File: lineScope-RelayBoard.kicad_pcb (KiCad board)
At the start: 2 copper layers, 99.5 x 38 mm, 18 parts, among them J10 Conn_01x03, J2 Conn_01x02, K1 RM85-1011-35-1012, K2 RM85-1011-35-1012, K3 RM85-1011-35-1012

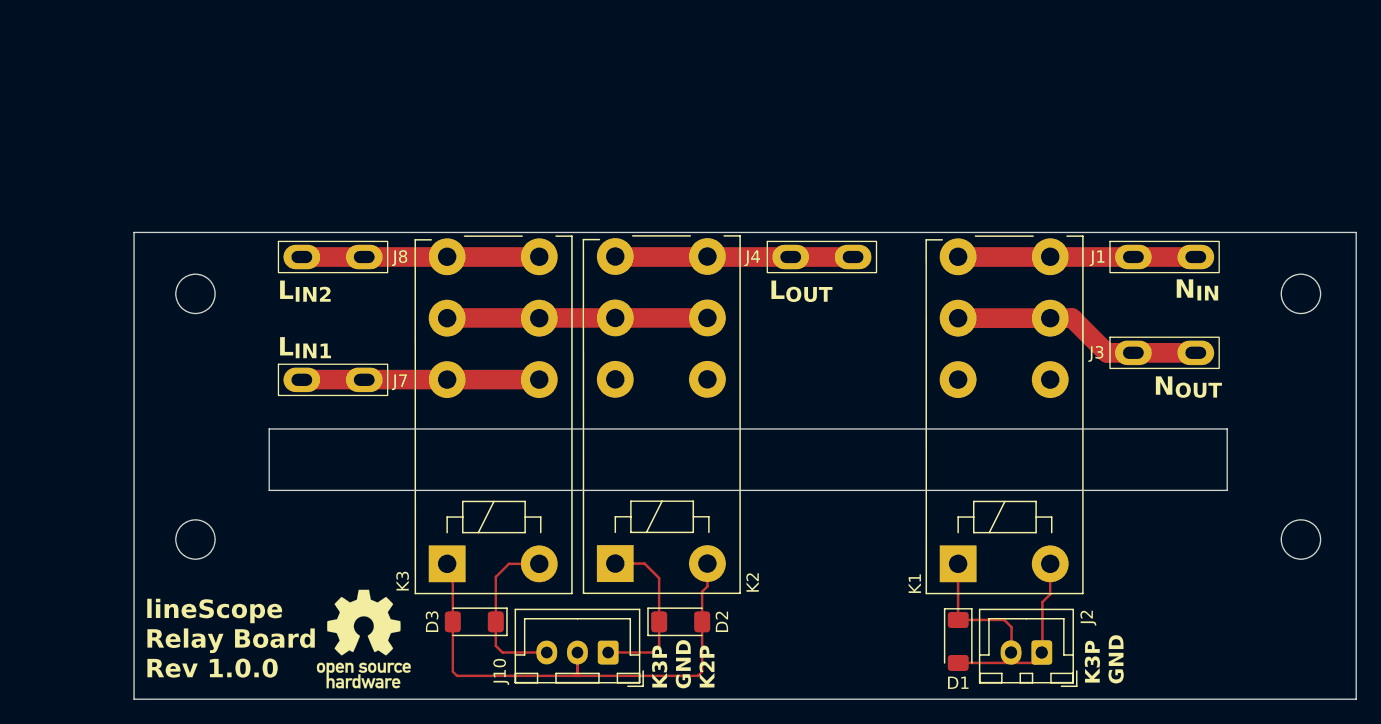
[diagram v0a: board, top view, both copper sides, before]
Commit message: Minor fixes
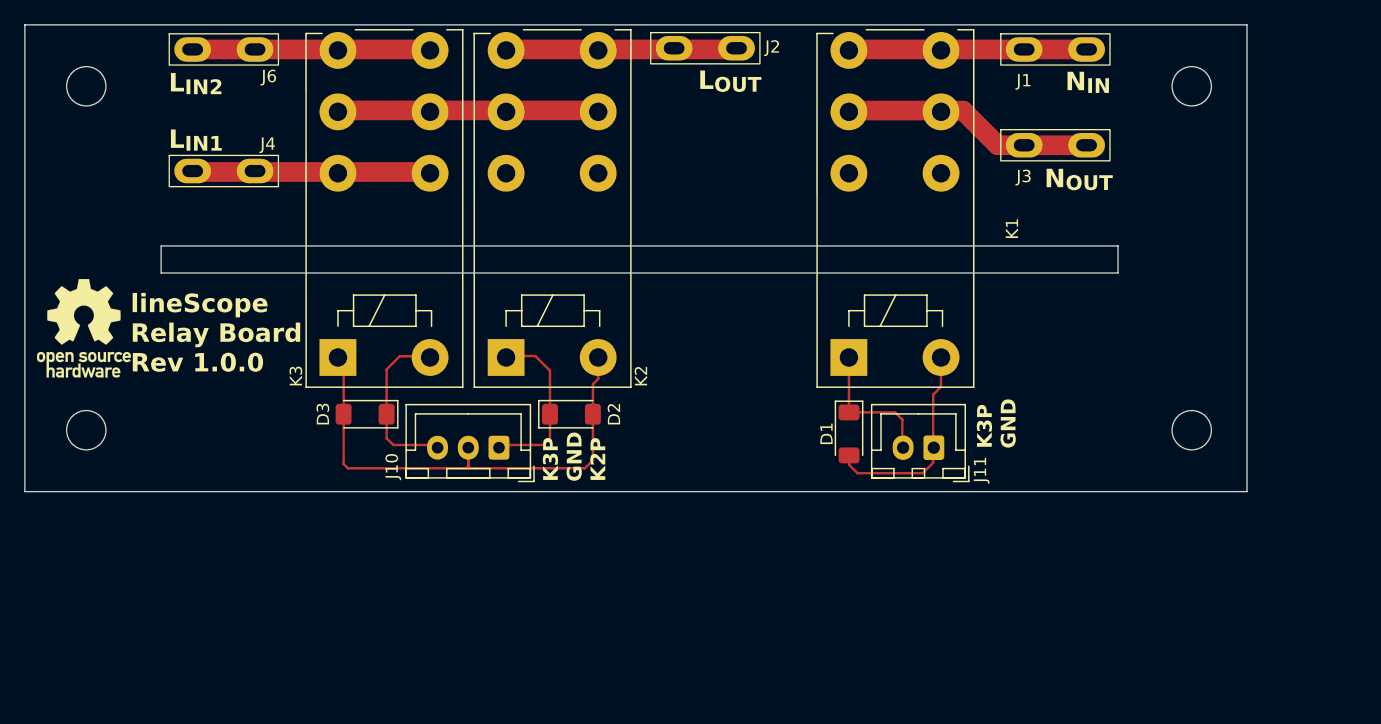
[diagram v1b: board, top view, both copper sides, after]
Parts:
- removed J7, J8: ~, Koszalix_Connectors_Tab:TE-1-726388-2
- added J11: Conn_01x02, Connector_JST:JST_XH_B2B-XH-A_1x02_P2.50mm_Vertical, F.Cu at (172.1, 90.5)
- added J6: ~, Koszalix_Connectors_Tab:TE-1-726388-2, F.Cu at (114.3, 58.1)
- J2: value Conn_01x02 -> ~; footprint Connector_JST:JST_XH_B2B-XH-A_1x02_P2.50mm_Vertical -> Koszalix_Connectors_Tab:TE-1-726388-2
- K1, K2, K3: footprint Koszalix_Relays:RM84 -> Koszalix_Relays:RM85_Socket
- moved J2 56.3 mm to (153.5, 58.0), turned to 0 degrees
- moved J4 49.2 mm to (114.3, 68.0)
- moved REF** 34.1 mm to (102.9, 80.8)
- moved J1 19.1 mm to (182.0, 58.1)
- moved H4 19.1 mm to (103.1, 61.1)
- moved J3 19.1 mm to (182.0, 65.9)
- moved D2 19.1 mm to (142.6, 87.8)
- moved D3 19.1 mm to (125.8, 87.8)
- moved H2 19.1 mm to (193.1, 61.1)
- moved D1 19.1 mm to (165.2, 89.4)
- moved K1 19.0 mm to (169.0, 72.1)
- moved K3 19.0 mm to (127.4, 72.1)
- moved K2 19.0 mm to (141.1, 72.1)
- moved J10 18.9 mm to (136.7, 90.5)
- moved H3 12.6 mm to (103.1, 89.1)
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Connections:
- J2 pad 1: /K1GND -> /HV.L_{OUT}
- J4 pad 1: /HV.L_{OUT} -> /HV.L_{IN_{1}}
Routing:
- net /K1GND: track 14.9 -> 17.2 mm
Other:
- outline, holes or cut-outs redrawn
- board text added: "0"
- board text added: "0 mm"
- board text added: "0,0000 mm / 0,0000 mm"
- board text added: "0,01 mm"
- board text added: "0,02"
- board text added: "0,035 mm"
- board text added: "0,3000 mm"
- board text added: "1"
- board text added: "1,51 mm"
- board text added: "1,6000 mm"
- board text added: "2"
- board text added: "3,3"
- board text added: "4,5"
- board text added: "99,5000 mm x 38,0000 mm"
- board text added: "B.Cu"
- board text added: "B.Mask"
- board text added: "B.Paste"
- board text added: "B.Silkscreen"
- board text added: "BOARD CHARACTERISTICS"
- board text added: "Board Thickness:"
- board text added: "Board overall dimensions:"
- board text added: "Bottom Silk Screen"
- board text added: "Bottom Solder Mask"
- board text added: "Bottom Solder Paste"
- board text added: "Castellated pads:"
- board text added: "Color"
- board text added: "Copper Finish:"
- board text added: "Copper Layer Count:"
- board text added: "Dielectric"
- board text added: "Edge card connectors:"
- board text added: "Epsilon R"
- board text added: "F.Cu"
- board text added: "F.Mask"
- board text added: "F.Paste"
- board text added: "F.Silkscreen"
- board text added: "FR4"
- board text added: "Impedance Control:"
- board text added: "Layer Name"
- board text added: "Loss Tangent"
- board text added: "Material"
- board text added: "Min hole diameter:"
- board text added: "Min track/spacing:"
- board text added: "No"
- board text added: "None"
- board text added: "Not specified"
- board text added: "Plated Board Edge:"
- board text added: "Thickness (mm)"
- board text added: "Top Silk Screen"
- board text added: "Top Solder Mask"
- board text added: "Top Solder Paste"
- board text added: "Type"
- board text added: "copper"
- board text added: "core"

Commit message: Update
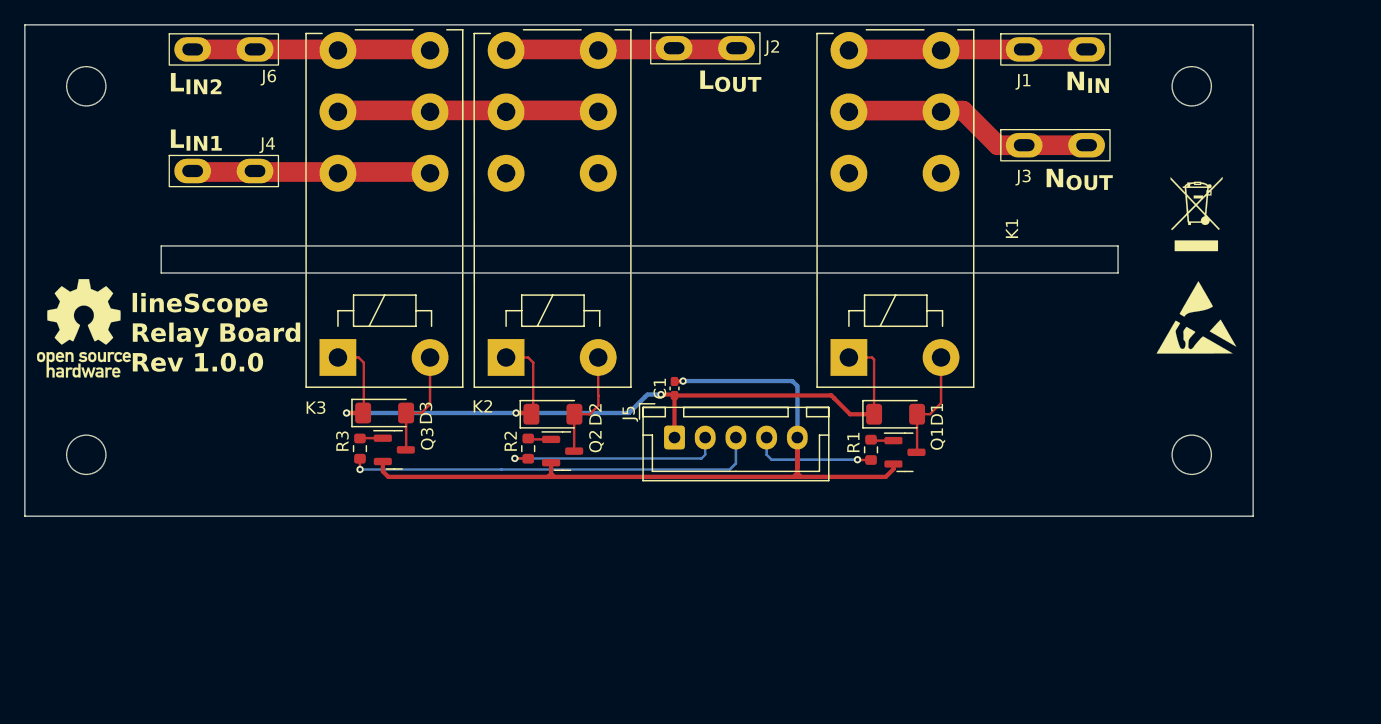
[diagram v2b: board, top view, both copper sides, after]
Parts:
- removed J10: Conn_01x03, Connector_JST:JST_XH_B3B-XH-A_1x03_P2.50mm_Vertical
- removed J11: Conn_01x02, Connector_JST:JST_XH_B2B-XH-A_1x02_P2.50mm_Vertical
- added C1: 100n, Capacitor_SMD:C_0402_1005Metric_Pad0.74x0.62mm_HandSolder, F.Cu at (151.0, 85.7)
- added J5: Conn_01x05, Connector_JST:JST_XH_B5B-XH-A_1x05_P2.50mm_Vertical, F.Cu at (151.0, 89.7)
- added Q1: BC847, Package_TO_SOT_SMD:SOT-23, F.Cu at (169.8, 90.9)
- added Q2: BC847, Package_TO_SOT_SMD:SOT-23, F.Cu at (141.9, 90.8)
- added Q3: BC847, Package_TO_SOT_SMD:SOT-23, F.Cu at (128.2, 90.7)
- added R1: 10k, Resistor_SMD:R_0603_1608Metric, F.Cu at (167.0, 90.7)
- added R2: 10k, Resistor_SMD:R_0603_1608Metric, F.Cu at (139.1, 90.6)
- added R3: 10k, Resistor_SMD:R_0603_1608Metric, F.Cu at (125.4, 90.6)
- added REF**: WEEE-Logo_4.2x6mm_SilkScreen, Symbol:WEEE-Logo_4.2x6mm_SilkScreen, F.Cu at (193.5, 71.5)
- added REF**: ESD-Logo_6.6x6mm_SilkScreen, Symbol:ESD-Logo_6.6x6mm_SilkScreen, F.Cu at (193.5, 79.9)
- moved D1 4.11 mm to (169.0, 87.8), turned to 0 degrees
- moved H1 2.00 mm to (193.1, 91.1)
- moved H3 2.00 mm to (103.1, 91.1)
- moved D3 1.59 mm to (127.4, 87.7), turned to 0 degrees
- moved D2 1.51 mm to (141.1, 87.8)
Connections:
- net /K1GND renamed Net-(D1-A)
- D1 pad 1: /K1PWR -> VCC
- D2 pad 1: /K2PWR -> VCC
- D2 pad 2: /K23GND -> Net-(D2-A)
- D3 pad 1: /K3PWR -> VCC
- D3 pad 2: /K23GND -> Net-(D3-A)
- K1 pad A1: /K1PWR -> VCC
- K2 pad A1: /K2PWR -> VCC
- K2 pad A2: /K23GND -> Net-(D2-A)
- K3 pad A1: /K23GND -> VCC
- K3 pad A2: /K3PWR -> Net-(D3-A)
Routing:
- net VCC: track 0.00 -> 70.7 mm, vias 0 -> 3
- net GND: track 0.00 -> 65.4 mm, vias 0 -> 1
- net /K23GND: track 42.8 -> 0.00 mm
- net /SEL: track 0.00 -> 33.8 mm, vias 0 -> 1
- net /L_{EN}: track 0.00 -> 18.1 mm, vias 0 -> 1
- net /K3PWR: track 14.0 -> 0.00 mm
- net /K2PWR: track 13.9 -> 0.00 mm
- net /K1PWR: track 10.4 -> 0.00 mm
- net /N_{EN}: track 0.00 -> 10.1 mm, vias 0 -> 1
- net Net-(D2-A): track 0.00 -> 9.29 mm
- net Net-(D3-A): track 0.00 -> 9.07 mm
- net Net-(D1-A): track 17.2 -> 9.16 mm
- net Net-(Q2-B): track 0.00 -> 1.89 mm
- net Net-(Q3-B): track 0.00 -> 1.87 mm
- net Net-(Q1-B): track 0.00 -> 1.86 mm
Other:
- board size 99.5 x 38 mm -> 100 x 40 mm
- board text added: "100,5000 mm x 40,0000 mm"
- board text removed: "99,5000 mm x 38,0000 mm"
- board text removed: "K3P GND"
- board text removed: "K3P GND K2P"
